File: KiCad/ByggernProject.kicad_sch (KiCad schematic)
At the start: 16 parts, among them J1 AVR-JTAG-10, SW1 SW_Push, U1 LATCH, U2 L7805, U3 MAX232, U5 SRAM, U6 ATmega162-16P

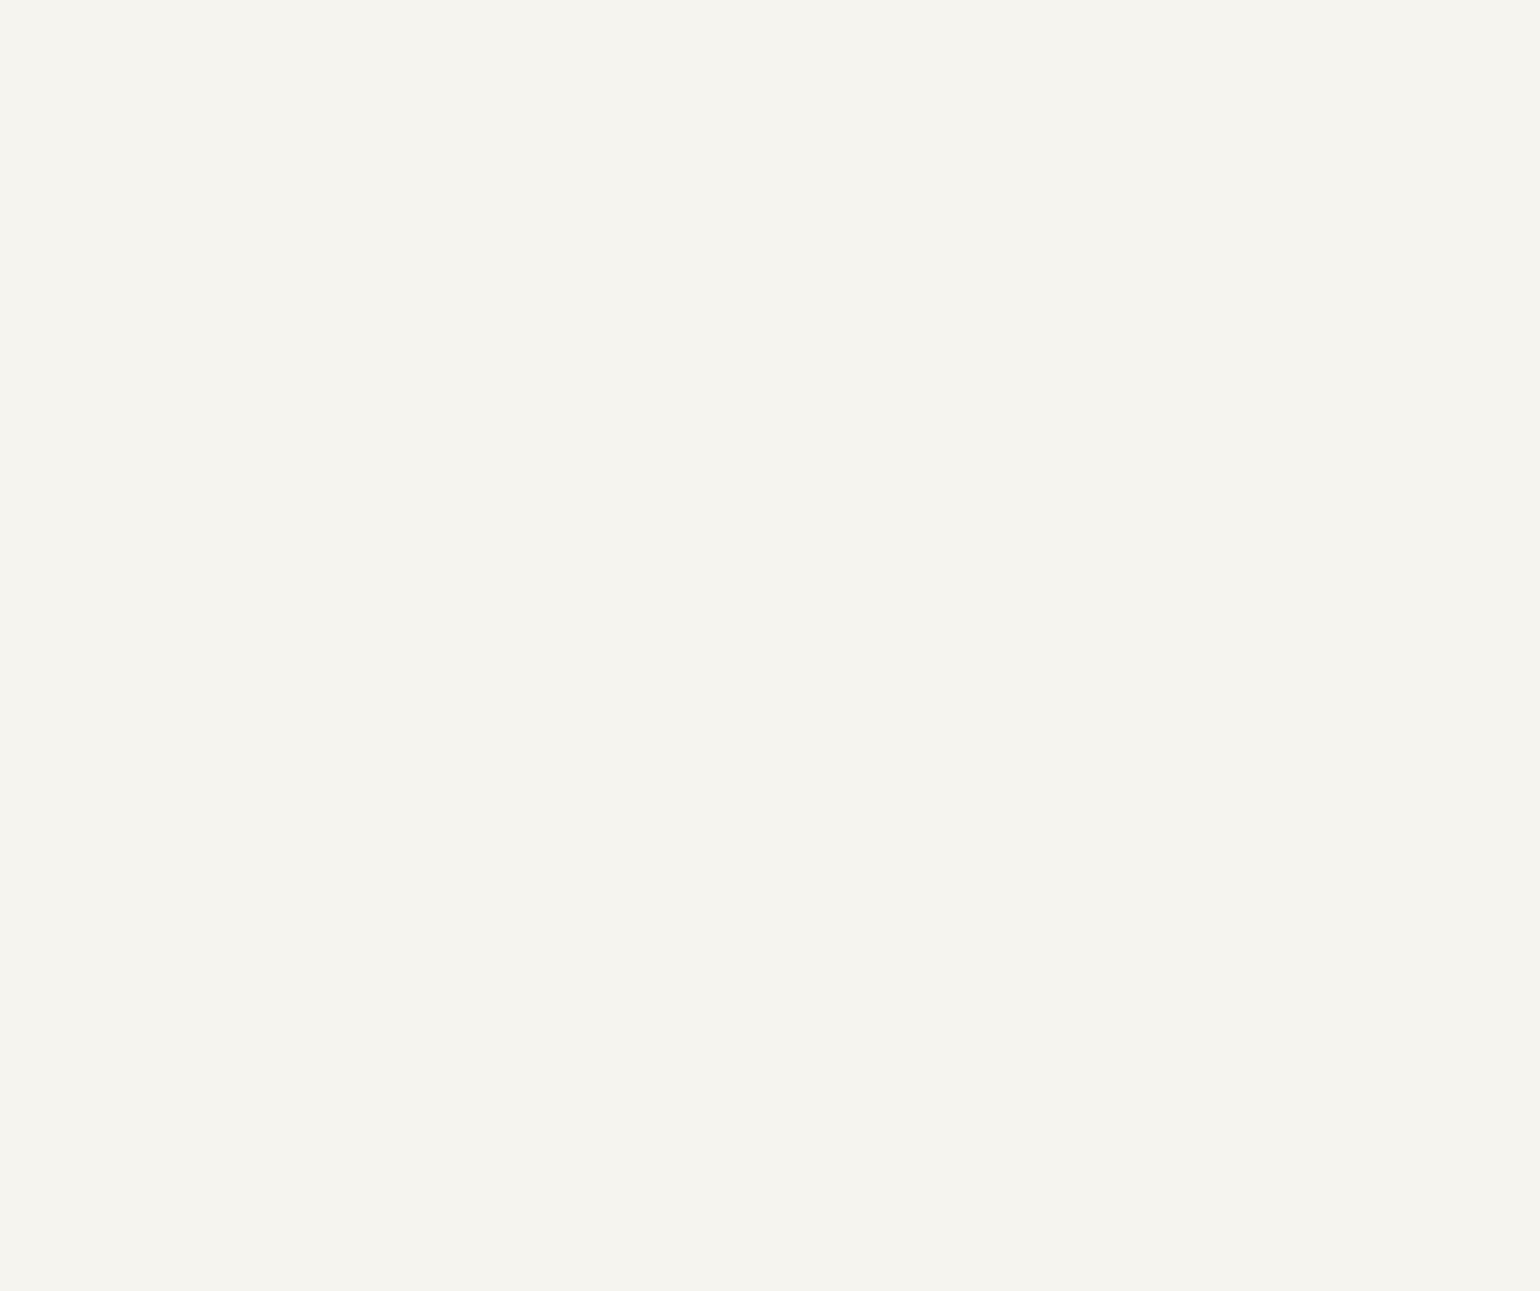
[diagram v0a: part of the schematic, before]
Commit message: uPPDADED KEYCAD
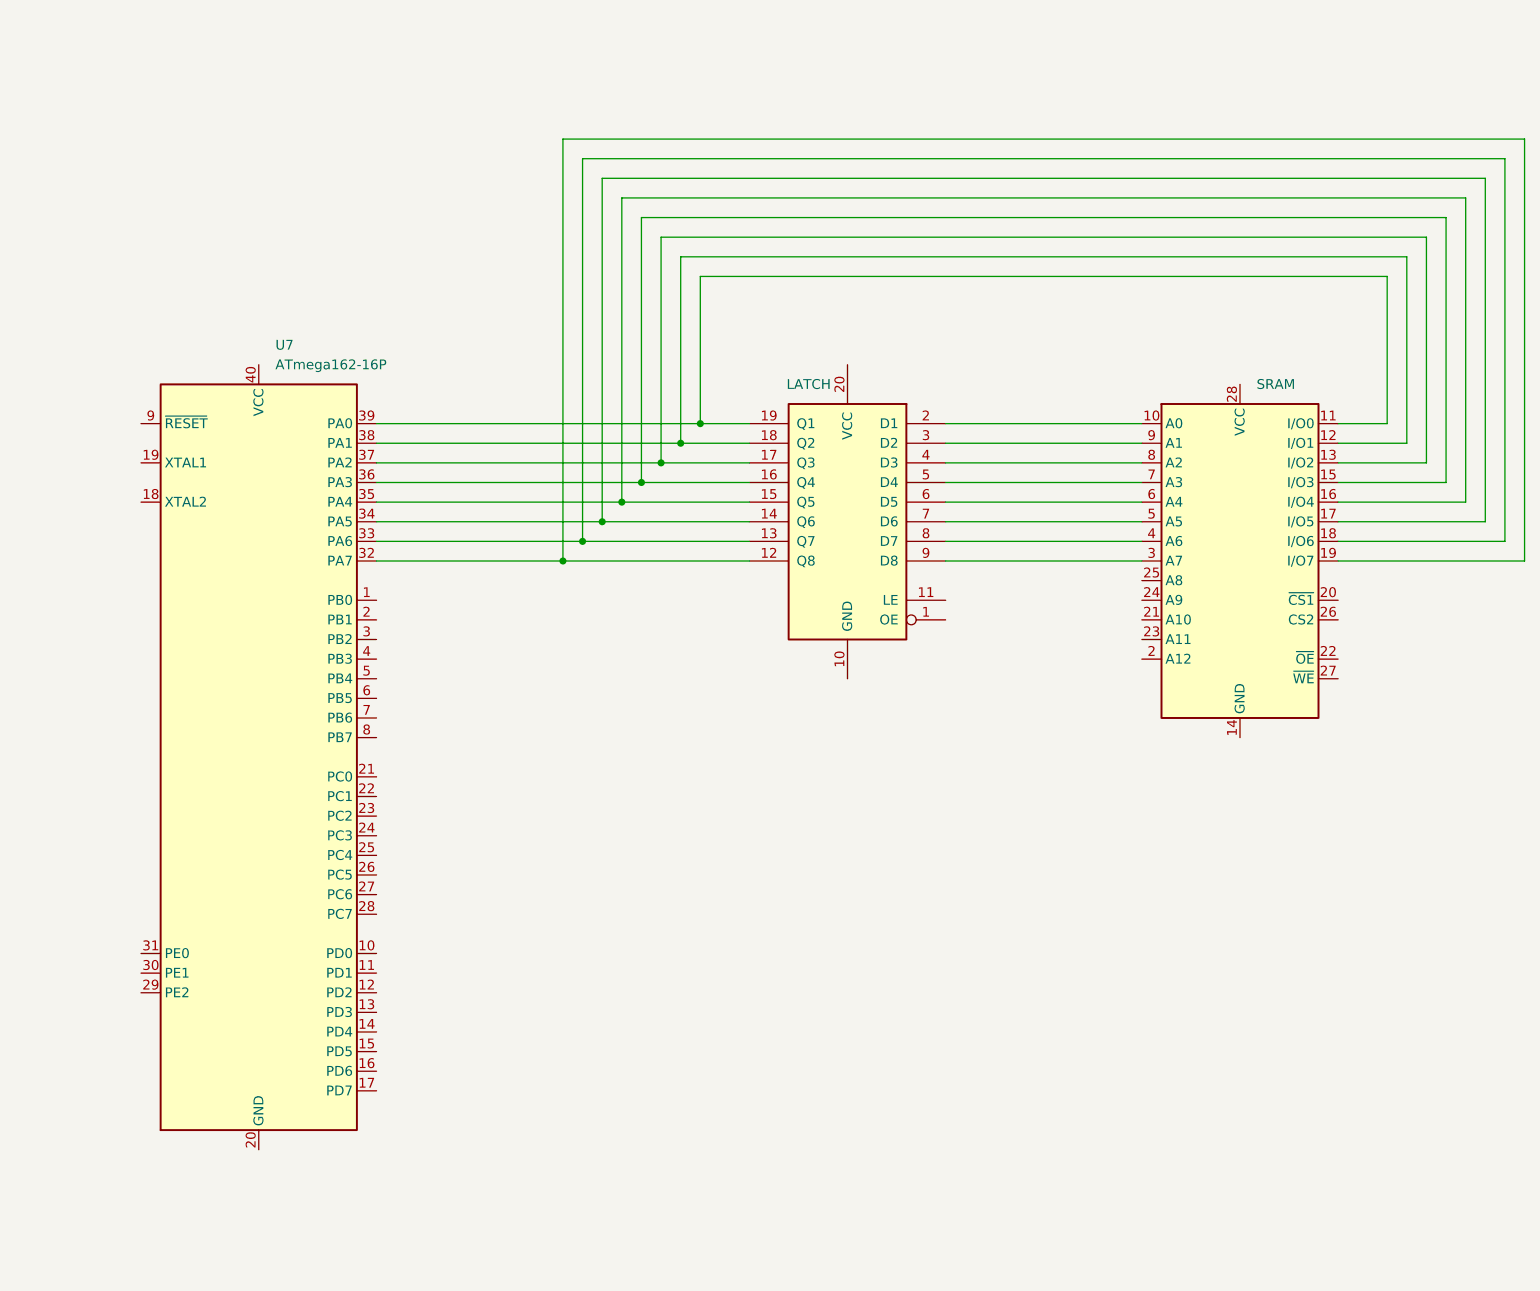
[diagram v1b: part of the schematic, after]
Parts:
- added U4: LATCH, symbol 74xx:74LS573
- added U7: ATmega162-16P, Package_DIP:DIP-40_W15.24mm, symbol MCU_Microchip_ATmega:ATmega162-16P
- added U8: SRAM, Package_SO:SOP-28_8.4x18.16mm_P1.27mm, symbol Memory_RAM:HY6264AxJ
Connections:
- new net: U4.12 (Q8), U7.32 (PA7), U8.19 (I/O7)
- new net: U4.13 (Q7), U7.33 (PA6), U8.18 (I/O6)
- new net: U4.14 (Q6), U7.34 (PA5), U8.17 (I/O5)
- new net: U4.15 (Q5), U7.35 (PA4), U8.16 (I/O4)
- new net: U4.16 (Q4), U7.36 (PA3), U8.15 (I/O3)
- new net: U4.17 (Q3), U7.37 (PA2), U8.13 (I/O2)
- new net: U4.18 (Q2), U7.38 (PA1), U8.12 (I/O1)
- new net: U4.19 (Q1), U7.39 (PA0), U8.11 (I/O0)
- new net: U4.2 (D1), U8.10 (A0)
- new net: U4.9 (D8), U8.3 (A7)
- new net: U4.8 (D7), U8.4 (A6)
- new net: U4.7 (D6), U8.5 (A5)
- new net: U4.6 (D5), U8.6 (A4)
- new net: U4.5 (D4), U8.7 (A3)
- new net: U4.4 (D3), U8.8 (A2)
- new net: U4.3 (D2), U8.9 (A1)
